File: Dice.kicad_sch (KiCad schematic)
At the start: 24 parts, among them Q1 NPN, SW1 SW_Push, U1 LM555xM, U2 4017, U3 74LS32

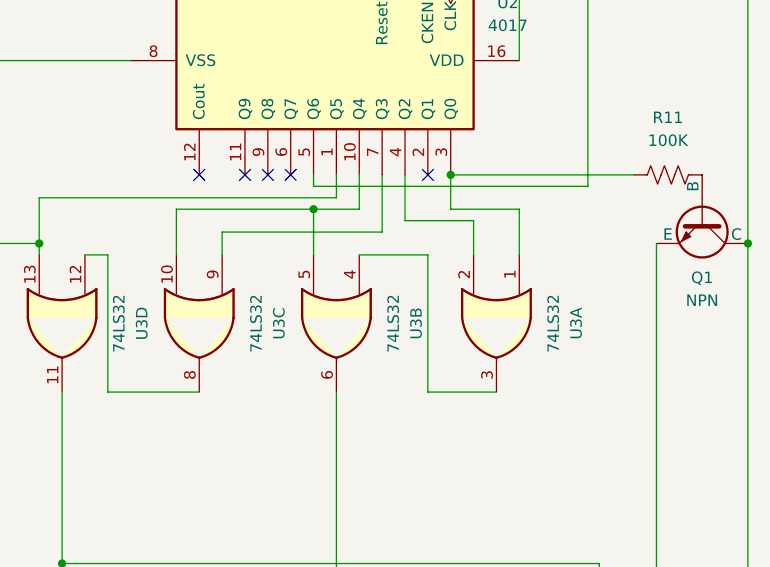
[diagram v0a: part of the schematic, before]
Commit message: test
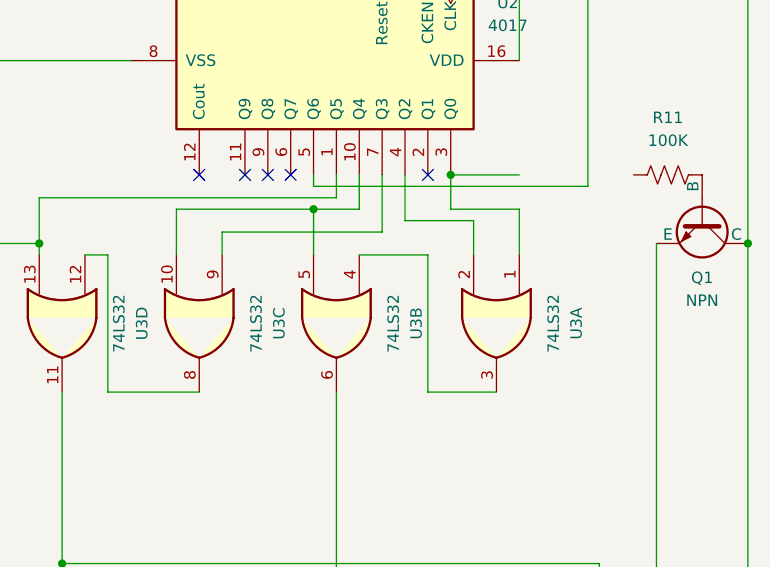
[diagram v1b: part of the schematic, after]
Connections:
- net at U2.3 (Q0), U3.1: no longer R11.1
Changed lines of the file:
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@@
 	(paper "A4")
 	(junction
+		(at 111.76 99.06)
+		(diameter 0)
+		(color 0 0 0 0)
+	)
+	(junction
 		(at 160.02 140.97)
 		(diameter 0)
@@
 	(junction
 		(at 127 62.23)
-		(diameter 0)
-		(color 0 0 0 0)
-	)
-	(junction
-		(at 111.76 99.06)
 		(diameter 0)
 		(color 0 0 0 0)
@@
 	(wire
 		(pts
+			(xy 96.52 99.06) (xy 111.76 99.06)
+		)
+		(stroke
+			(width 0)
+			(type default)
+		)
+	)
+	(wire
+		(pts
 			(xy 114.3 97.79) (xy 81.28 97.79)
 		)
@@
 	(wire
 		(pts
-			(xy 111.76 99.06) (xy 96.52 99.06)
-		)
-		(stroke
-			(width 0)
-			(type default)
-		)
-	)
-	(wire
-		(pts
 			(xy 104.14 156.21) (xy 129.54 156.21)
 		)
@@
 	(wire
 		(pts
-			(xy 132.08 119.38) (xy 124.46 119.38)
+			(xy 124.46 119.38) (xy 132.08 119.38)
 		)
 		(stroke
@@
 	(wire
 		(pts
-			(xy 127 95.25) (xy 147.32 95.25)
-		)
-		(stroke
+			(xy 127 95.25) (xy 134.62 95.25)
+		)
+		(stroke

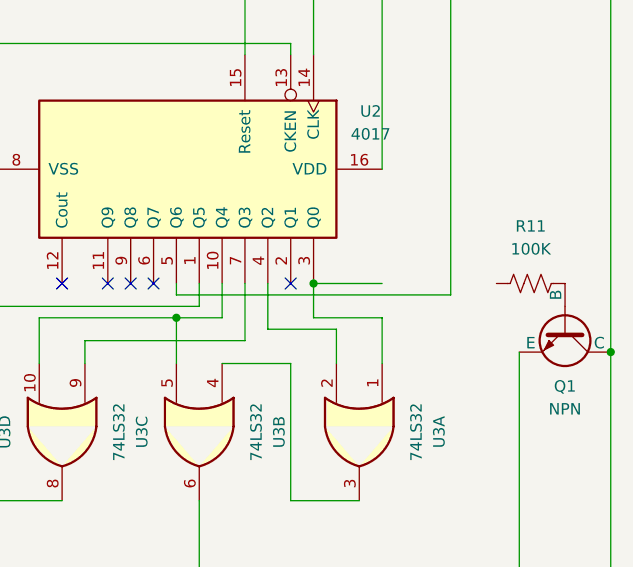
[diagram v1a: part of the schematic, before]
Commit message: test
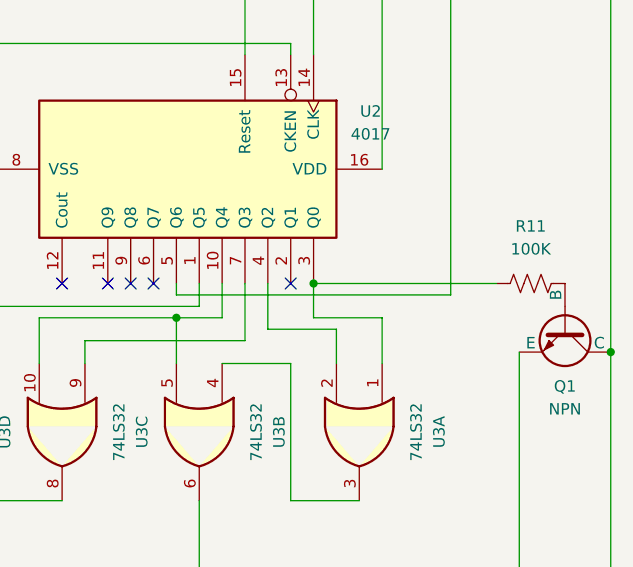
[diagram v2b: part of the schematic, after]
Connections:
- net at R11.1: now also U2.3 (Q0), U3.1
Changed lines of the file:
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@@
 	(wire
 		(pts
-			(xy 127 95.25) (xy 134.62 95.25)
+			(xy 127 95.25) (xy 147.32 95.25)
 		)
 		(stroke
